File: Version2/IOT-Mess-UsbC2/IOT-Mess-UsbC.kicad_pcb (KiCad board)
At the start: 2 copper layers, 22.3 x 18.3 mm, 16 parts, among them J1 Conn_01x04_Pin, J2 Jumper_2, J3 Conn_01x04_Pin, J4 Jumper_2, J5 Jumper_2, U1 USB_C_Receptacle_USB2.0_16P, U2 ME6211C33M5

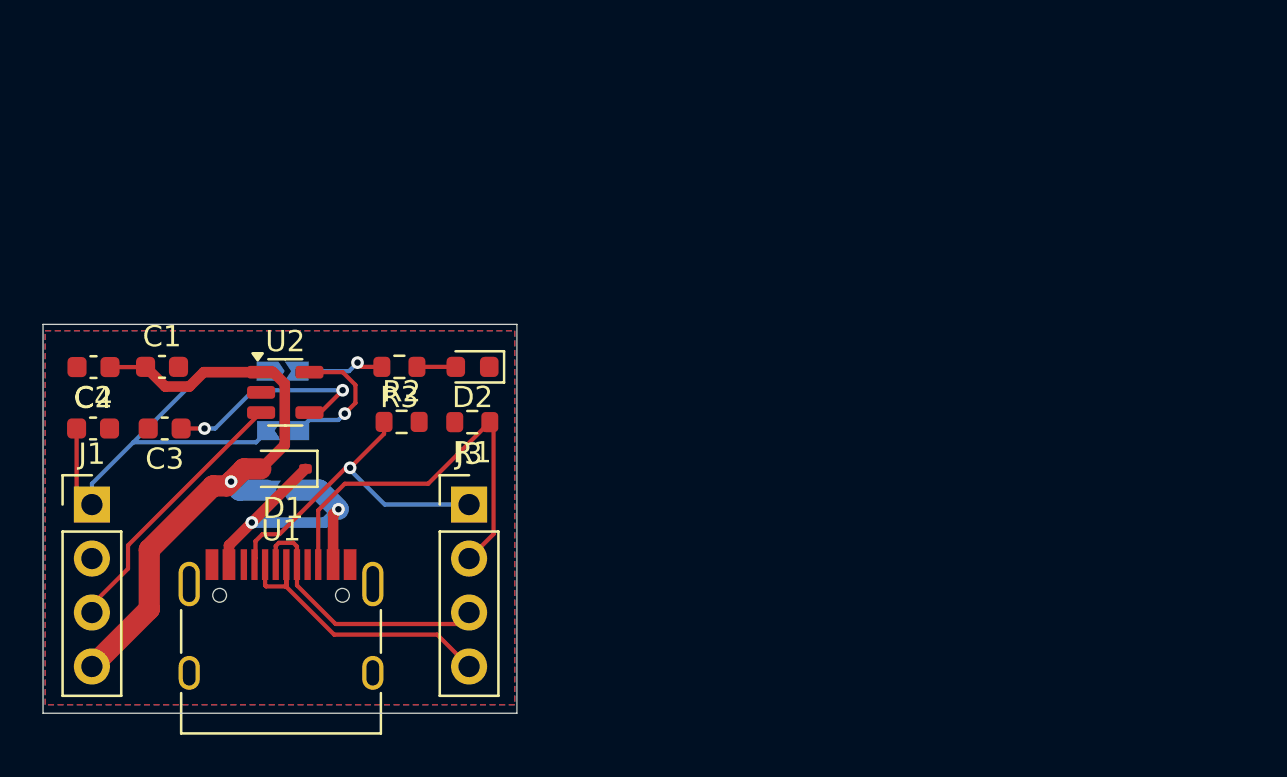
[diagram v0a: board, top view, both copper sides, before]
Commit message: added jumper boards.
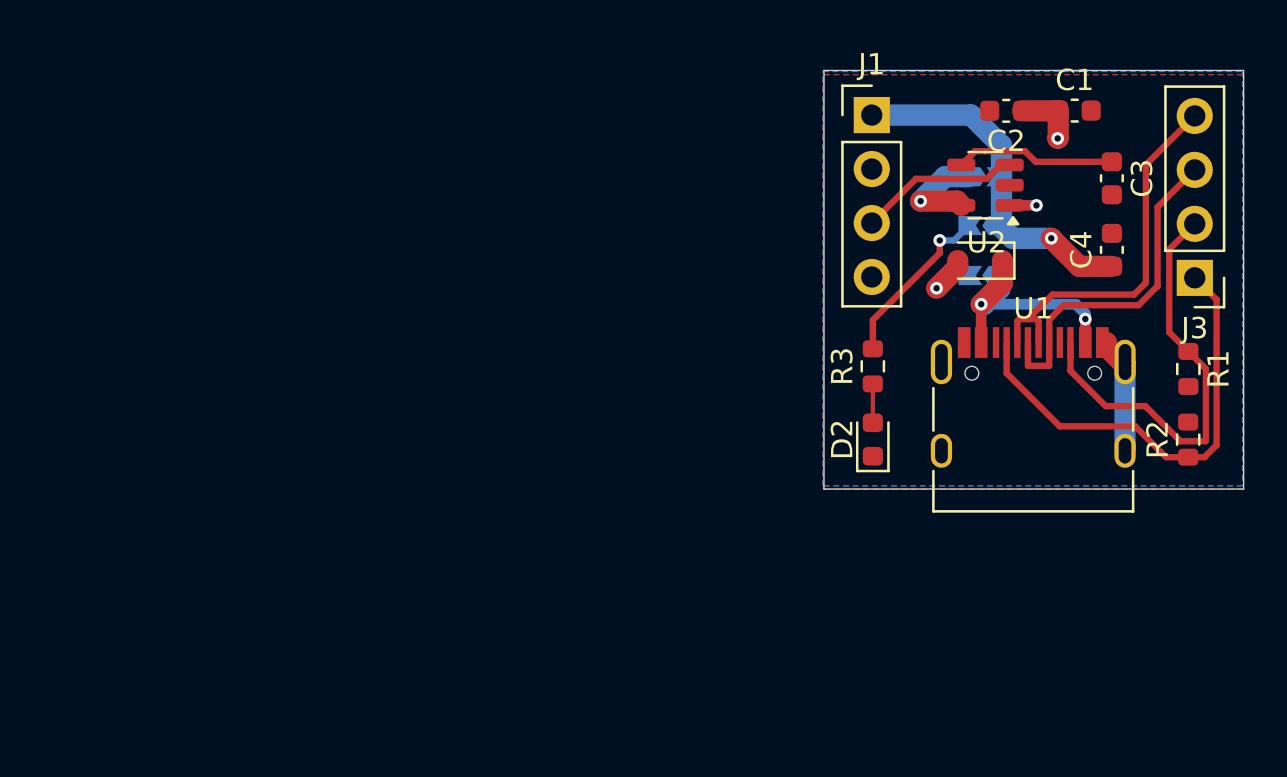
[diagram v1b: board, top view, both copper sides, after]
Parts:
- moved C4 48.7 mm to (188.5, 108.9), turned to 90 degrees
- moved C3 46.1 mm to (188.5, 105.5), turned to -90 degrees
- moved C2 44.6 mm to (183.5, 102.3)
- moved C1 44.6 mm to (186.8, 102.3)
- moved J1 41.0 mm to (177.2, 102.5)
- moved R2 37.0 mm to (192.1, 117.8), turned to 90 degrees
- moved U1 36.9 mm to (184.8, 117.3)
- moved J3 35.8 mm to (192.4, 110.2), turned to 180 degrees
- moved J4 35.1 mm to (182.5, 105.5), turned to 0 degrees
- moved J2 34.5 mm to (182.5, 110.1)
- moved U2 34.4 mm to (182.6, 105.8), turned to 180 degrees
- moved D1 34.2 mm to (182.3, 109.4)
- moved R1 33.8 mm to (192.1, 114.5), turned to -90 degrees
- moved J5 33.7 mm to (182.5, 107.8), turned to 180 degrees
- moved R3 22.3 mm to (177.2, 114.4), turned to 90 degrees
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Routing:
- net 5V: track 28.8 -> 5.98 mm, vias 1 -> 3
- net GND: track 0.16 -> 5.55 mm
- net CC1: track 16.2 -> 21.5 mm, vias 1 -> 0
- net +3.3V: track 21.8 -> 16.6 mm, vias 0 -> 1
- net CE: track 12.7 -> 7.62 mm
- net D-: track 14.2 -> 18.2 mm
- net Net-(J5-B): track 4.27 -> 8.07 mm
- net D+: track 12.9 -> 16.2 mm
- net Net-(D1-K): track 15.5 -> 12.5 mm
- net Net-(U2-NC): track 10.3 -> 7.56 mm, vias 2 -> 0
- net Net-(J4-A): track 6.48 -> 4.75 mm
- net CC2: track 19.3 -> 20.5 mm
- added copper zone on B.Cu, net 5V
- removed copper zone on B.Cu, net GND
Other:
- board size 22.3 x 18.3 mm -> 19.8 x 19.7 mm
